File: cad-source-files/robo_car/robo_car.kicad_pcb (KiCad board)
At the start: 2 copper layers, 100 x 100 mm, 91 parts, among them J1 Conn_01x06_MountingPin, J16 Conn_01x02_MountingPin, J2 ftdi_conn, J3 Conn_01x06_MountingPin, J4 Barrel_Jack, J5 Conn_01x04, J6 Conn_01x06_MountingPin, J7 Conn_01x02_MountingPin, J8 Conn_01x02_MountingPin, SW1 SW_Push, SW2 SW_Push, U1 XL1509, U2 AMS1117-3.3, U3 ESP32-WROOM-32U, U4 MOTOR_DRIVER-LV8548MC-AH

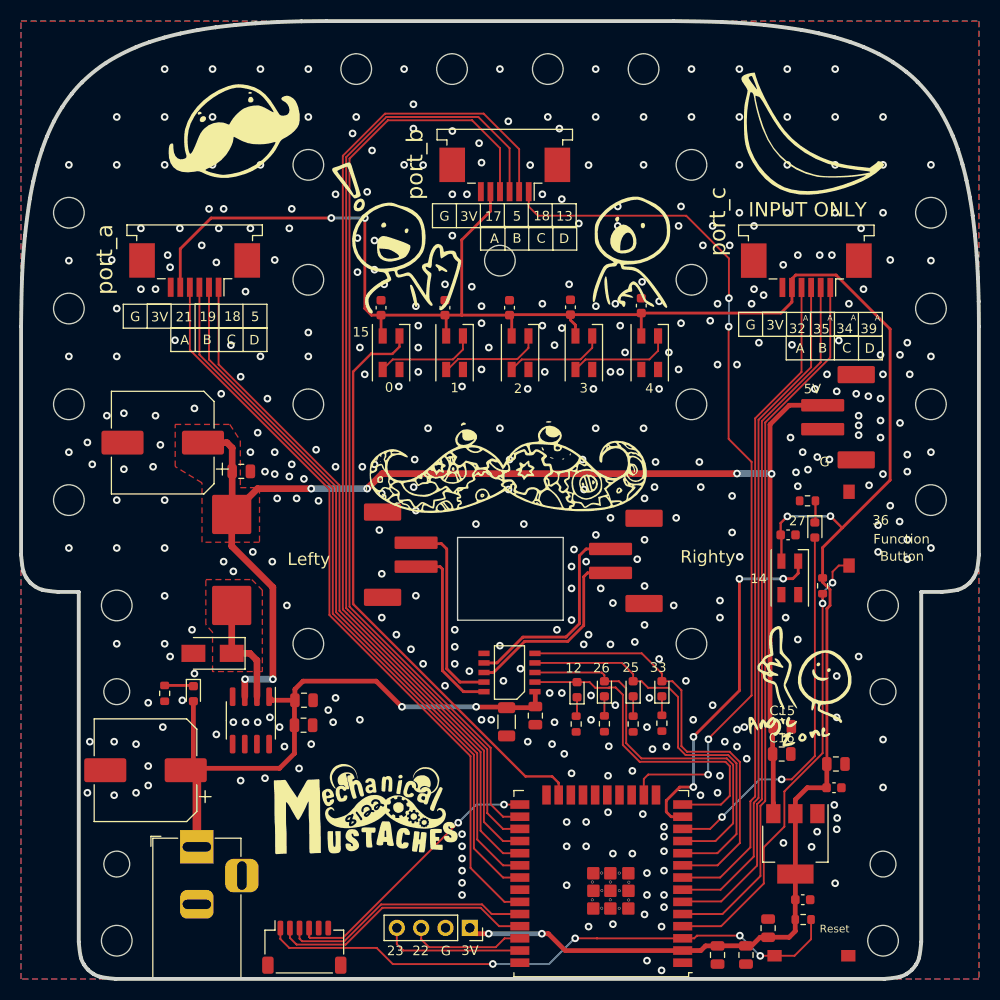
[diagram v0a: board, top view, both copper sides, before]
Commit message: squiggly squiggly
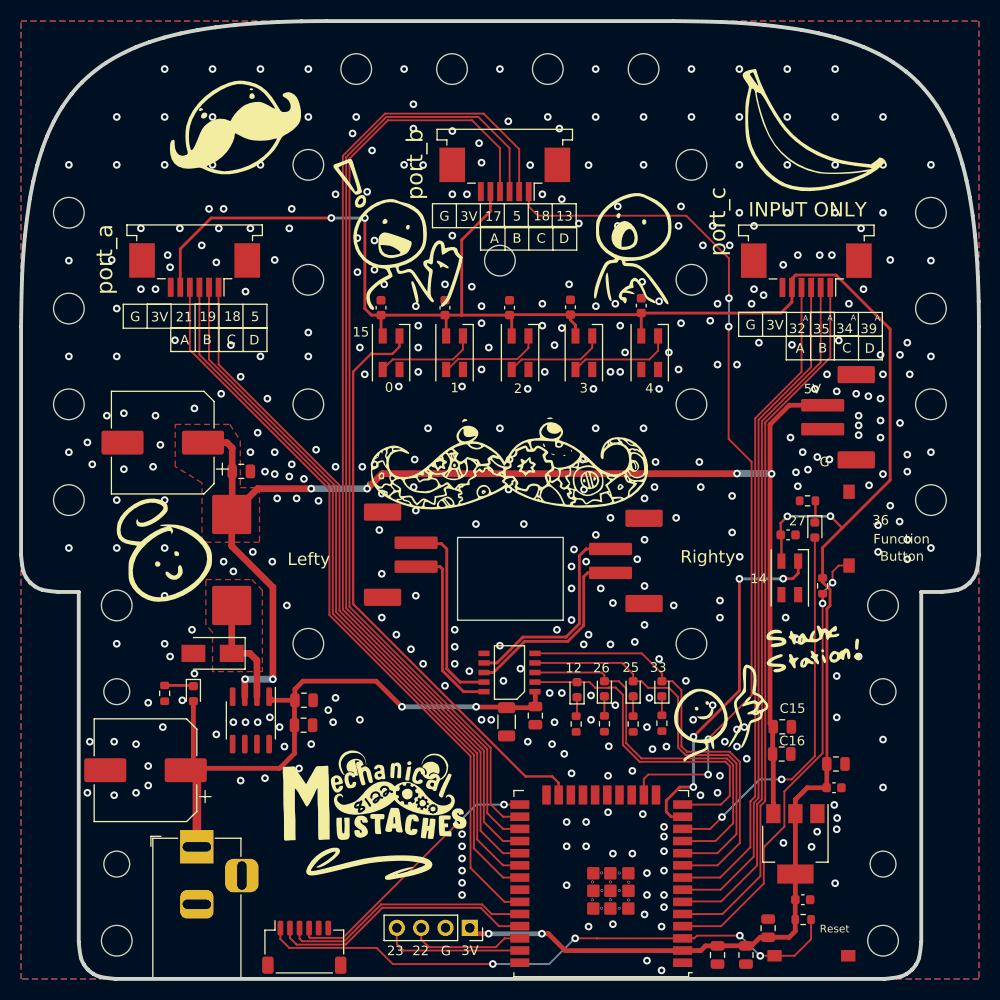
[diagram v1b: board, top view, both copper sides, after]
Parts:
- removed the G*** at (150.8, 101.3)
- added G***: LOGO, Symbol:Squiggly, F.Cu at (150.3, 98.4)
- added G***: LOGO, Symbol:Smiley, F.Cu at (150.6, 104.0)
- added G***: LOGO, Symbol:MustacheSS, F.Cu at (150.9, 100.9)
- added G***: LOGO, Symbol:stache_station, F.Cu at (152.4, 102.3)
- moved G*** 1.69 mm to (136.8, 131.5)
